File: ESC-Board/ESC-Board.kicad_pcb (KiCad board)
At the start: 2 copper layers, 17.1 x 32 mm, 4 parts

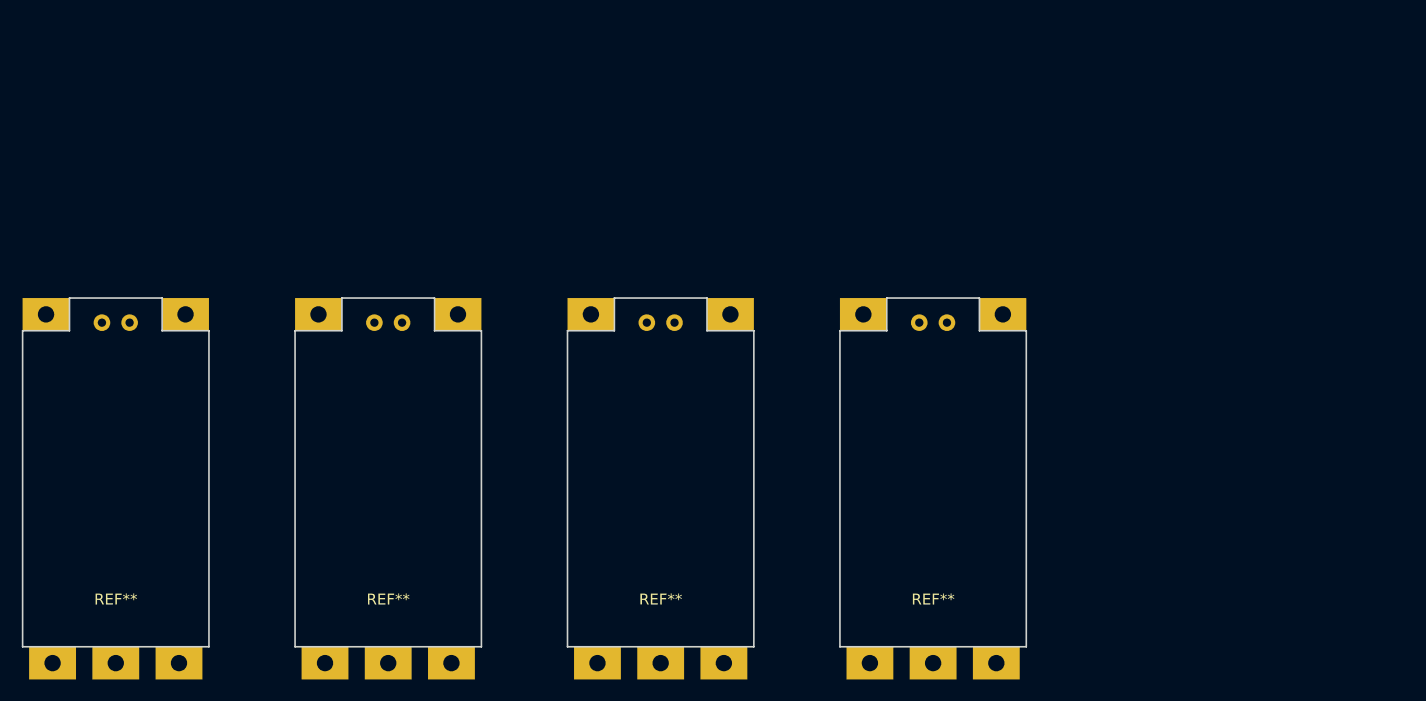
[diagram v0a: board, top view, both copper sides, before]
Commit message: Final Draft(with net list)
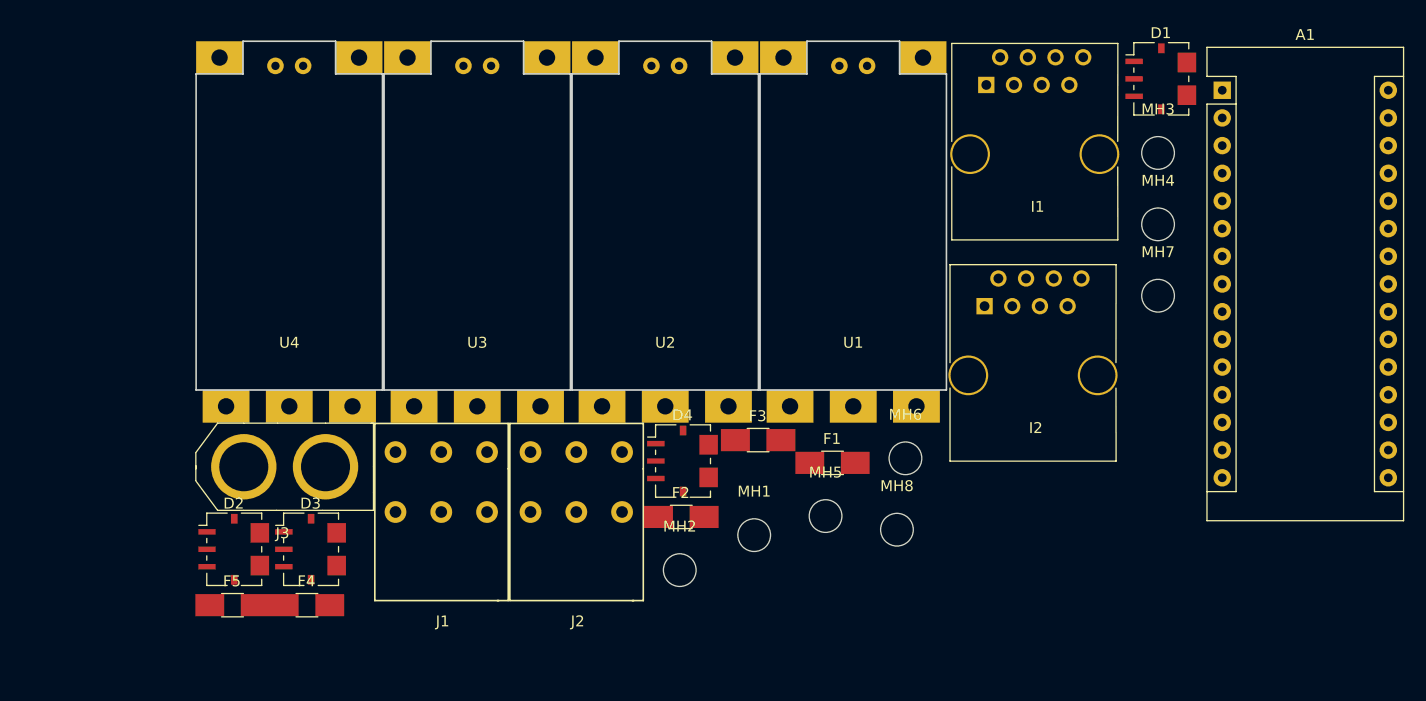
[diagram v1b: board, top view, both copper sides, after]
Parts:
- removed REF** (x4): Blue_ESC, Blue_ESC:Blue_ESC
- added A1: Arduino_Nano_v3.x, Blue_ESC:Arduino_Nano, F.Cu at (176.5, 43.4)
- added D1: ACS780xLRTR-100U, Blue_ESC:Allegro_PSOF-7_4.8x6.4mm_Pitch1.60mm, F.Cu at (170.9, 42.4)
- added D2: ACS780xLRTR-100U, Blue_ESC:Allegro_PSOF-7_4.8x6.4mm_Pitch1.60mm, F.Cu at (85.8, 85.6)
- added D3: ACS780xLRTR-100U, Blue_ESC:Allegro_PSOF-7_4.8x6.4mm_Pitch1.60mm, F.Cu at (92.9, 85.6)
- added D4: ACS780xLRTR-100U, Blue_ESC:Allegro_PSOF-7_4.8x6.4mm_Pitch1.60mm, F.Cu at (127.0, 77.5)
- added F1: 10/15, Fuse_Holders_and_Fuses:Fuse_SMD1206_HandSoldering, F.Cu at (140.8, 77.6)
- added F2: 10/15, Fuse_Holders_and_Fuses:Fuse_SMD1206_HandSoldering, F.Cu at (126.9, 82.6)
- added F3: 10/15, Fuse_Holders_and_Fuses:Fuse_SMD1206_HandSoldering, F.Cu at (133.9, 75.5)
- added F4: 10/15, Fuse_Holders_and_Fuses:Fuse_SMD1206_HandSoldering, F.Cu at (92.5, 90.7)
- added F5: 500m, Fuse_Holders_and_Fuses:Fuse_SMD1206_HandSoldering, F.Cu at (85.7, 90.7)
- added I1: RJ45, Connectors:RJ45_8, F.Cu at (154.9, 42.9)
- added I2: RJ45, Connectors:RJ45_8, F.Cu at (154.7, 63.2)
- added J1: Molex, Blue_ESC:Molex_6pin, F.Cu at (104.9, 82.1)
- added J2: Molex, Blue_ESC:Molex_6pin, F.Cu at (117.3, 82.1)
- added J3: XT_60, Blue_ESC:XT60, F.Cu at (86.7, 78.0)
- added MH1: MountingHole, Mounting_Holes:MountingHole_3mm, F.Cu at (133.6, 84.3)
- added MH2: MountingHole, Mounting_Holes:MountingHole_3mm, F.Cu at (126.8, 87.5)
- added MH3: MountingHole, Mounting_Holes:MountingHole_3mm, F.Cu at (170.6, 49.2)
- added MH4: MountingHole, Mounting_Holes:MountingHole_3mm, F.Cu at (170.6, 55.7)
- added MH5: MountingHole, Mounting_Holes:MountingHole_3mm, F.Cu at (140.1, 82.5)
- added MH6: MountingHole, Mounting_Holes:MountingHole_3mm, F.Cu at (147.5, 77.2)
- added MH7: MountingHole, Mounting_Holes:MountingHole_3mm, F.Cu at (170.6, 62.3)
- added MH8: MountingHole, Mounting_Holes:MountingHole_3mm, F.Cu at (146.7, 83.8)
- added U1: ESC:Blue_ESC, Blue_ESC:Blue_ESC, F.Cu at (142.7, 56.4)
- added U2: ESC:Blue_ESC, Blue_ESC:Blue_ESC, F.Cu at (125.4, 56.4)
- added U3: ESC:Blue_ESC, Blue_ESC:Blue_ESC, F.Cu at (108.2, 56.4)
- added U4: ESC:Blue_ESC, Blue_ESC:Blue_ESC, F.Cu at (90.9, 56.4)

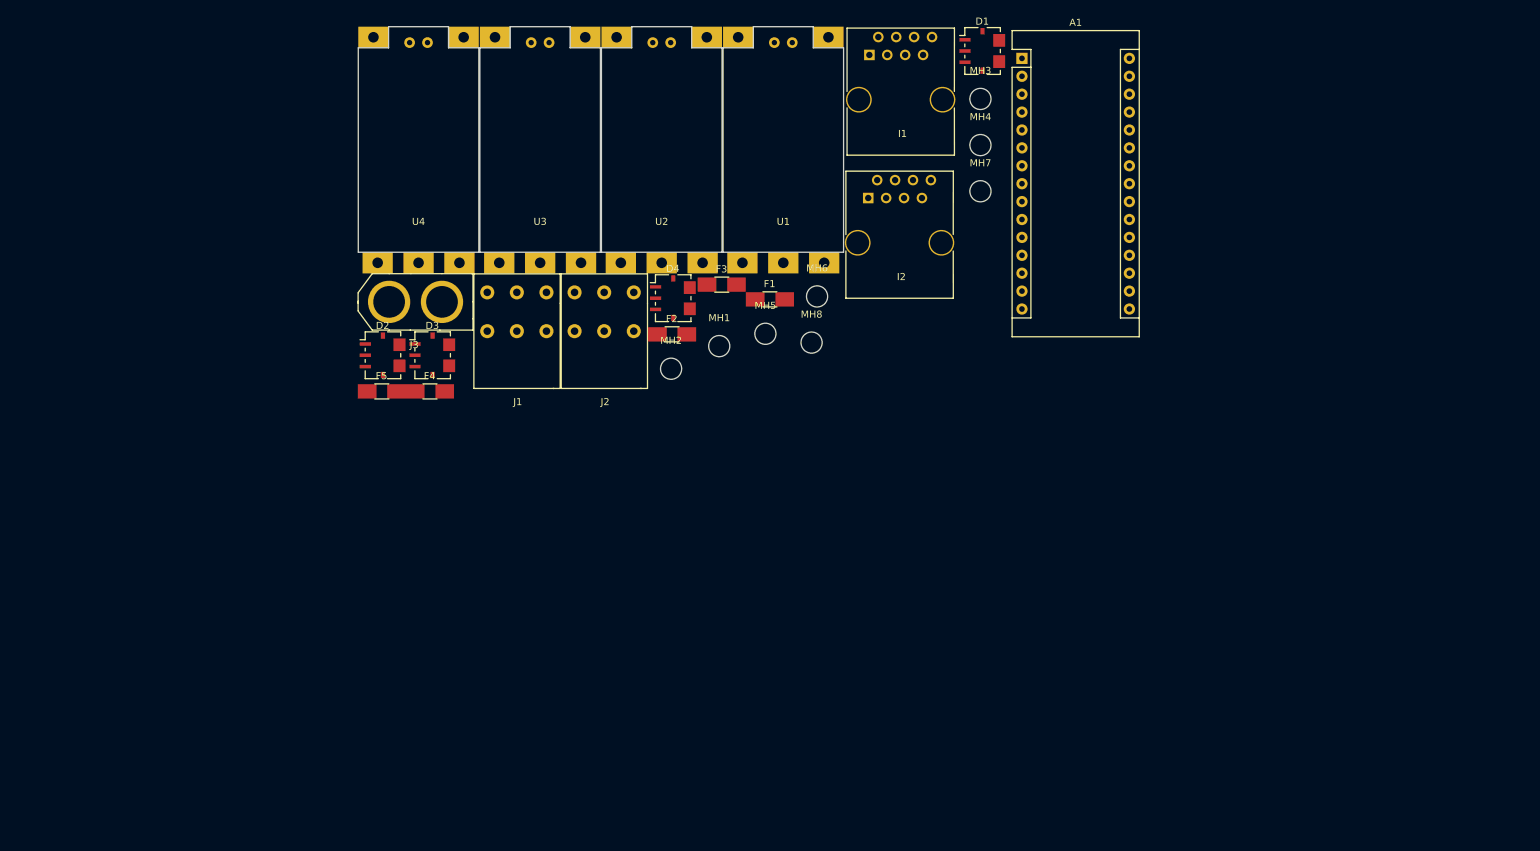
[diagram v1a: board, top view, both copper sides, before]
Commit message: Starting layout
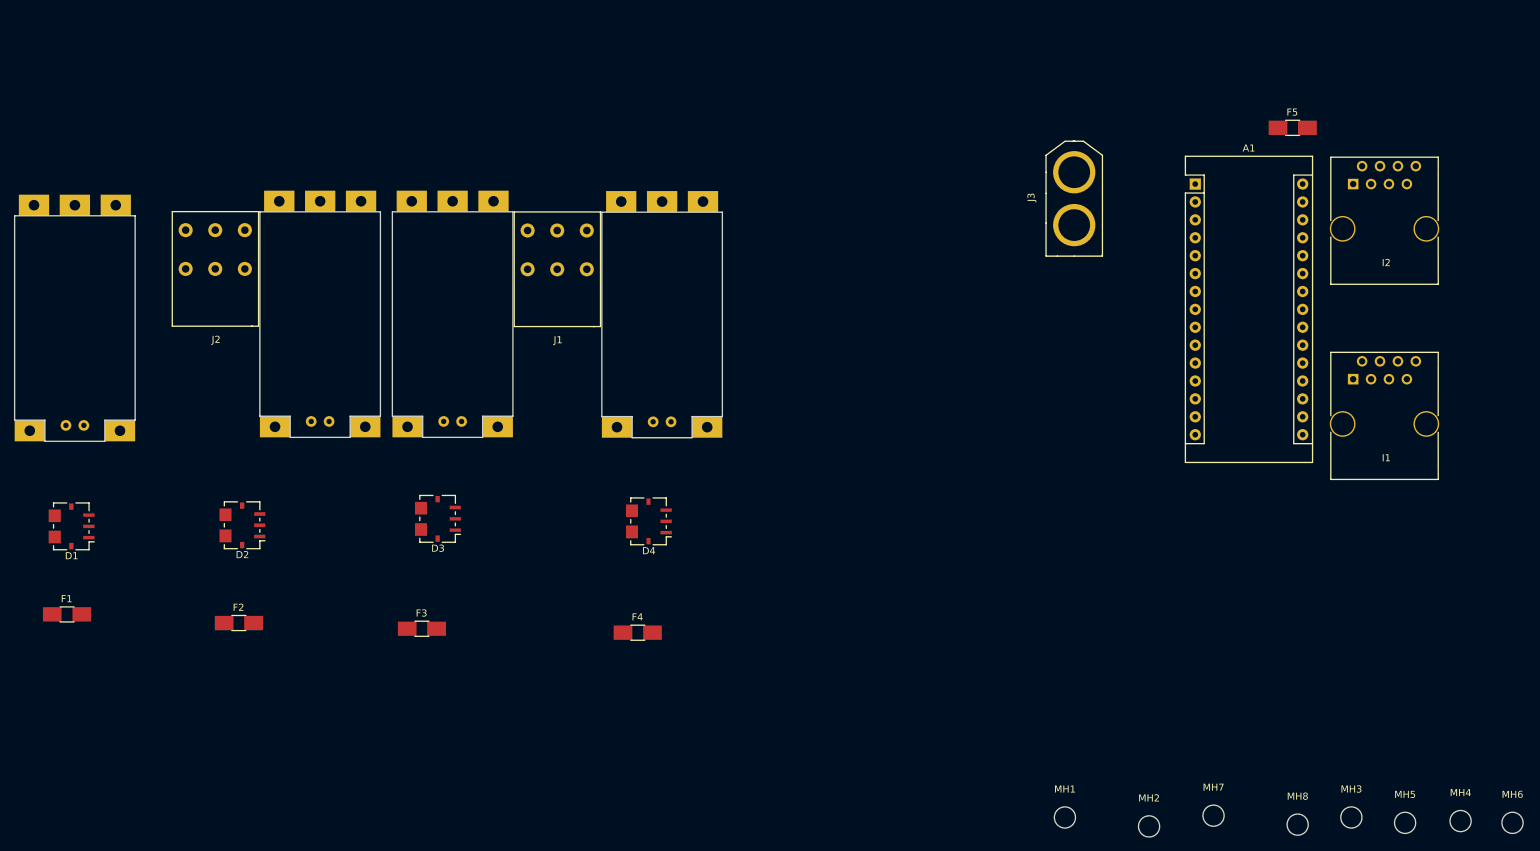
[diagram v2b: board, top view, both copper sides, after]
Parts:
- U1, U2, U3, U4: moved to B.Cu
- moved D1 145.7 mm to (41.7, 109.8), turned to 180 degrees
- moved F5 134.5 mm to (214.9, 53.3)
- moved MH6 123.7 mm to (246.1, 151.9)
- moved MH4 117.6 mm to (238.8, 151.6)
- moved MH3 114.7 mm to (223.3, 151.1)
- moved MH5 114.2 mm to (230.9, 151.9)
- moved F1 109.3 mm to (41.0, 122.3)
- moved U1 103.3 mm to (42.2, 80.3)
- moved J3 98.9 mm to (183.9, 59.6), turned to 270 degrees
- moved MH8 97.1 mm to (215.6, 152.1)
- moved MH7 94.6 mm to (203.7, 150.9)
- moved MH2 93.9 mm to (194.6, 152.4)
- moved MH1 82.9 mm to (182.6, 151.1)
- moved I1 82.6 mm to (223.5, 89.0)
- moved F2 73.9 mm to (65.4, 123.5)
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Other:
- outline, holes or cut-outs redrawn
